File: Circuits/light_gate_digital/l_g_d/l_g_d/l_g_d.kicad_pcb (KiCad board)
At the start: 2 copper layers, 37 x 29 mm, 12 parts, among them J1 Conn_01x03_Female, Q1 Q_Photo_NPN_CE, U1 LM393P

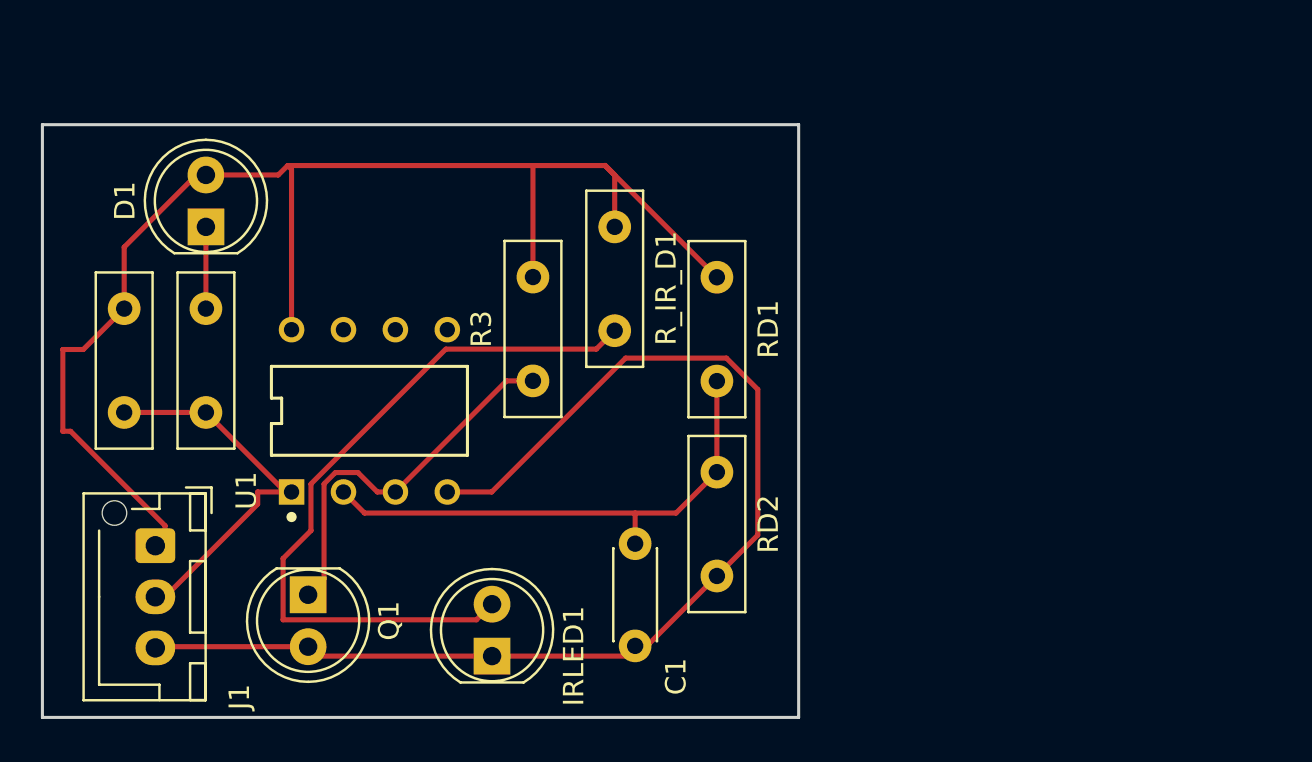
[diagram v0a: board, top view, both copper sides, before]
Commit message: --
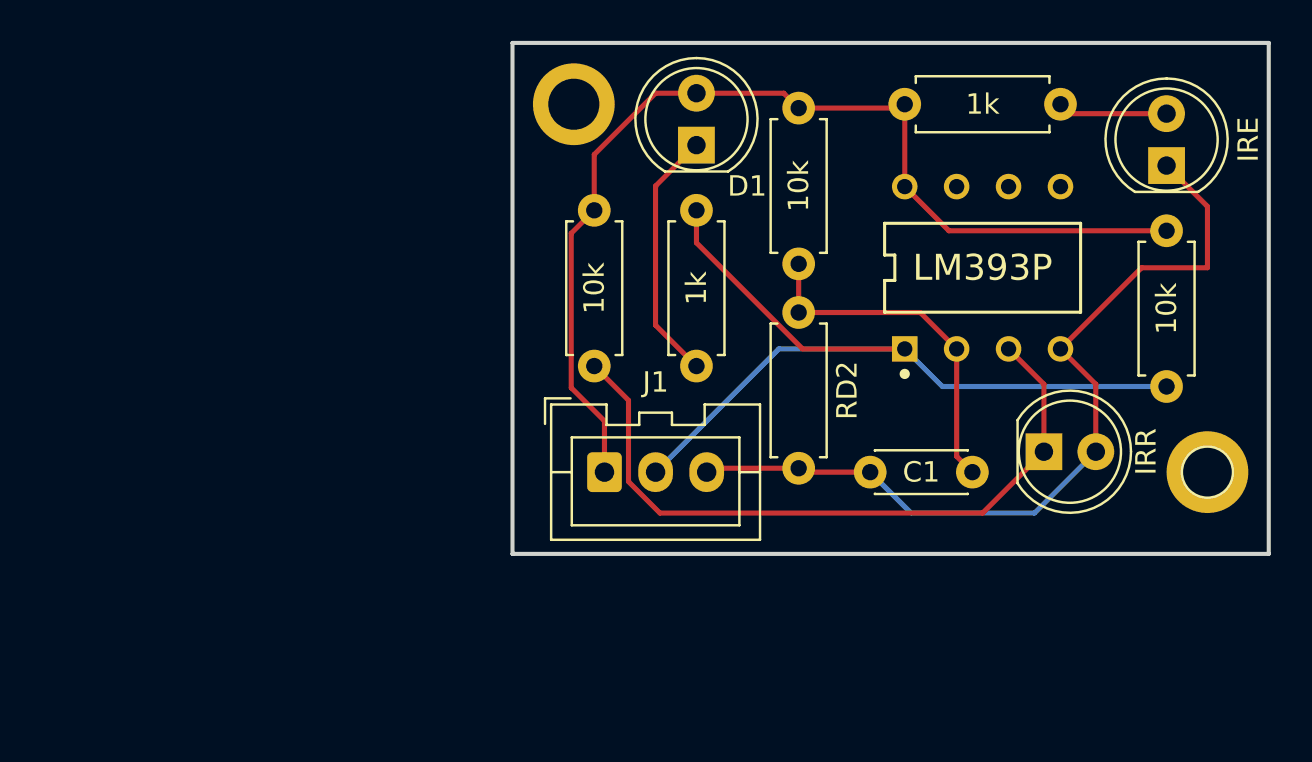
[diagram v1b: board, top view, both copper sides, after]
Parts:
- removed IRLED1: LD271, LED_THT:LED_D5.0mm_IRGrey
- removed Q1: Q_Photo_NPN_CE, LED_THT:LED_D5.0mm_IRGrey
- removed R3, R4, RD1: 10k, Resistor_THT:R_Box_L8.4mm_W2.5mm_P5.08mm
- removed R_D1, R_IR_D1: 1k, Resistor_THT:R_Box_L8.4mm_W2.5mm_P5.08mm
- added 10k: 10k, Resistor_THT:R_Axial_DIN0207_L6.3mm_D2.5mm_P7.62mm_Horizontal, F.Cu at (165.0, 61.2)
- added 10k: 10k, Resistor_THT:R_Axial_DIN0207_L6.3mm_D2.5mm_P7.62mm_Horizontal, F.Cu at (183.0, 67.2)
- added 10k: 10k, Resistor_THT:R_Axial_DIN0207_L6.3mm_D2.5mm_P7.62mm_Horizontal, F.Cu at (155.0, 73.8)
- added 1k: 1k, Resistor_THT:R_Axial_DIN0207_L6.3mm_D2.5mm_P7.62mm_Horizontal, F.Cu at (170.2, 61.0)
- added 1k: 1k, Resistor_THT:R_Axial_DIN0207_L6.3mm_D2.5mm_P7.62mm_Horizontal, F.Cu at (160.0, 73.8)
- added ?: , , F.Cu at (154.0, 61.0)
- added IRE: LD271, LED_THT:LED_D5.0mm_IRGrey, F.Cu at (183.0, 64.0)
- added IRR: Q_Photo_NPN_CE, LED_THT:LED_D5.0mm_IRGrey, F.Cu at (177.0, 78.0)
- added REF**: Pin_D1.0mm_L10.0mm, Connector_Pin:Pin_D1.0mm_L10.0mm, F.Cu at (185.0, 79.0)
- J1: footprint Connector_JST:JST_XH_B3B-XH-AM_1x03_P2.50mm_Vertical -> Connector_JST:JST_XA_B03B-XASK-1_1x03_P2.50mm_Vertical
- RD2: footprint Resistor_THT:R_Box_L8.4mm_W2.5mm_P5.08mm -> Resistor_THT:R_Axial_DIN0207_L6.3mm_D2.5mm_P7.62mm_Horizontal
- moved U1 30.8 mm to (174.0, 69.0)
- moved D1 24.3 mm to (160.0, 63.0)
- moved J1 22.3 mm to (155.5, 79.0), turned to 0 degrees
- moved C1 14.3 mm to (168.5, 79.0), turned to 0 degrees
- moved RD2 8.77 mm to (165.0, 71.2)
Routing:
- net Net-(IRLED1-Pad2): track 35.7 -> 5.38 mm
- net Net-(J1-Pad2): track 18.5 -> 42.2 mm
- net VCC: track 68.6 -> 51.2 mm
- net GND: track 57.3 -> 41.7 mm
- net Net-(Q1-Pad1): track 18.8 -> 34.3 mm
- net Net-(D1-Pad1): track 4.00 -> 12.5 mm
- net Net-(C1-Pad2): track 25.5 -> 17.2 mm
- added copper zone on B.Cu, net GND
- added copper zone on F.Cu, net GND
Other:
- board size 37 x 29 mm -> 37 x 25 mm
- board text added: "GND"
- board text added: "S"
- board text added: "VCC"
